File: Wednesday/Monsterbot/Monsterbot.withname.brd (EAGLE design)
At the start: 180 x 113 mm, 17 parts, among them U1_0_BRAIN ADAFRUIT-PRO-TRINKET-5V-BOB, U1_10_PENHOLDER_2 PENHOLDER, U1_11_PENHOLDER_3 PENHOLDER, U1_2_DISPLAY ADAFRUIT-1.2IN-8X8-LED-BACKPA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, U1_4_SERVO SERVOMICROSIDE, U1_5_CASTER CASTERADAFRUIT-3/4IN, U1_6_PENHOLDER PENHOLDER

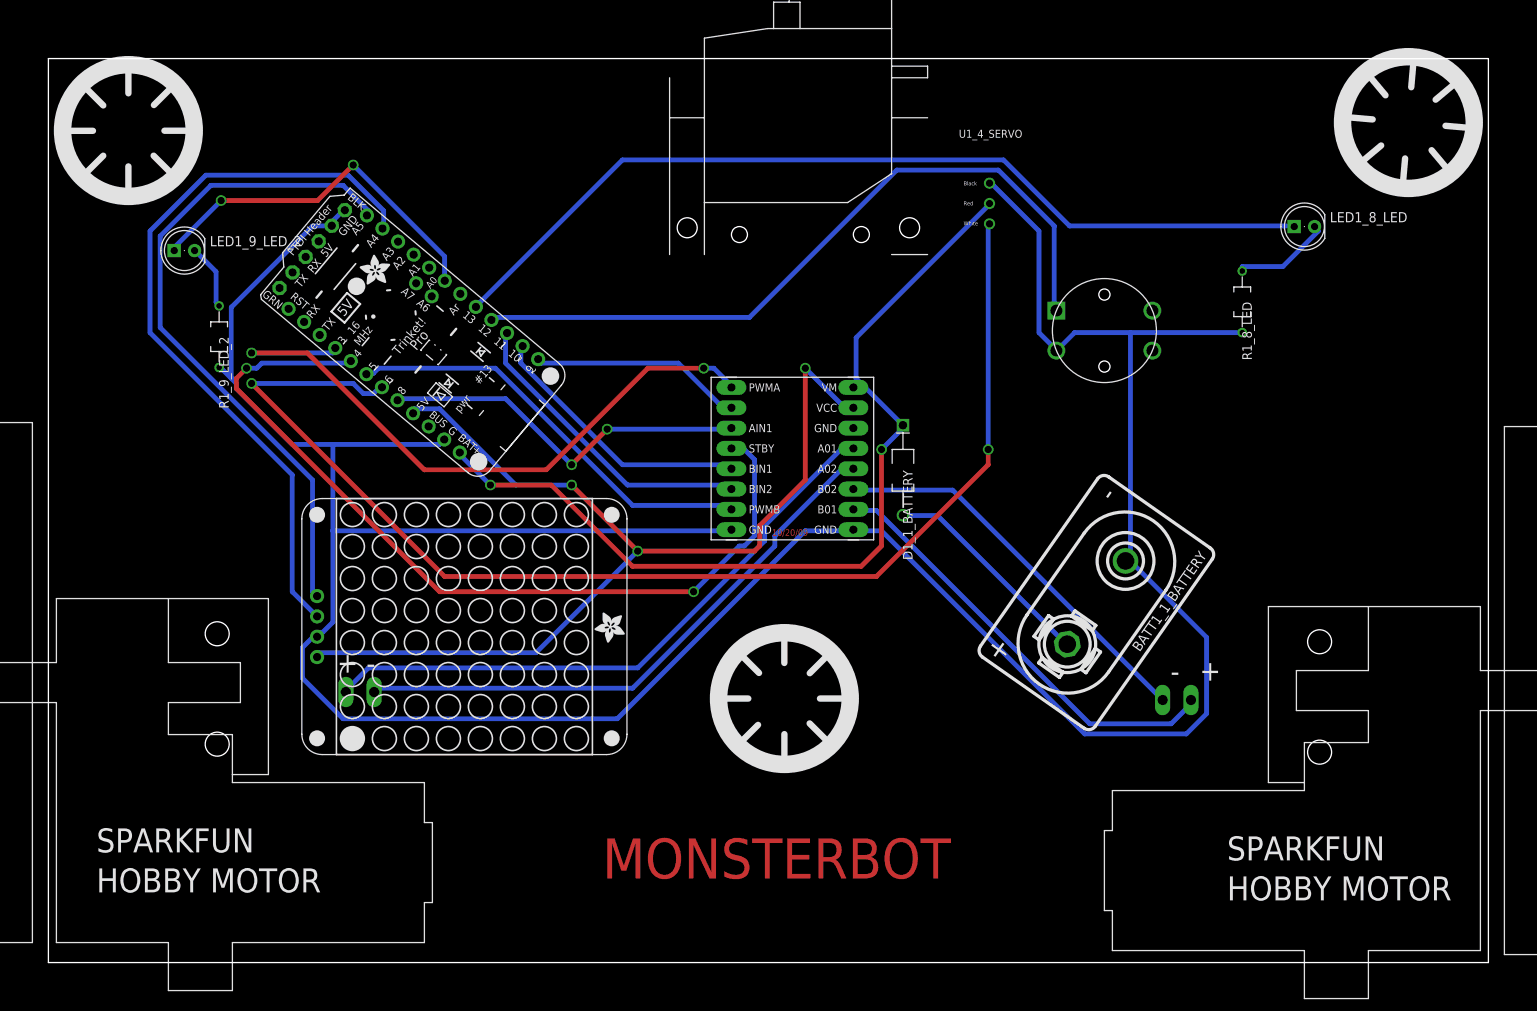
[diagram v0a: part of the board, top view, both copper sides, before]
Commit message: Readme
git-svn-id: svn+ssh://bbfs-01.calit2.net/grw/Gordon/svn/trunk/Gadgets/Designs/CSE91Robots@22925 2cf53259-273a-af40-bda6-69d31023b8ec
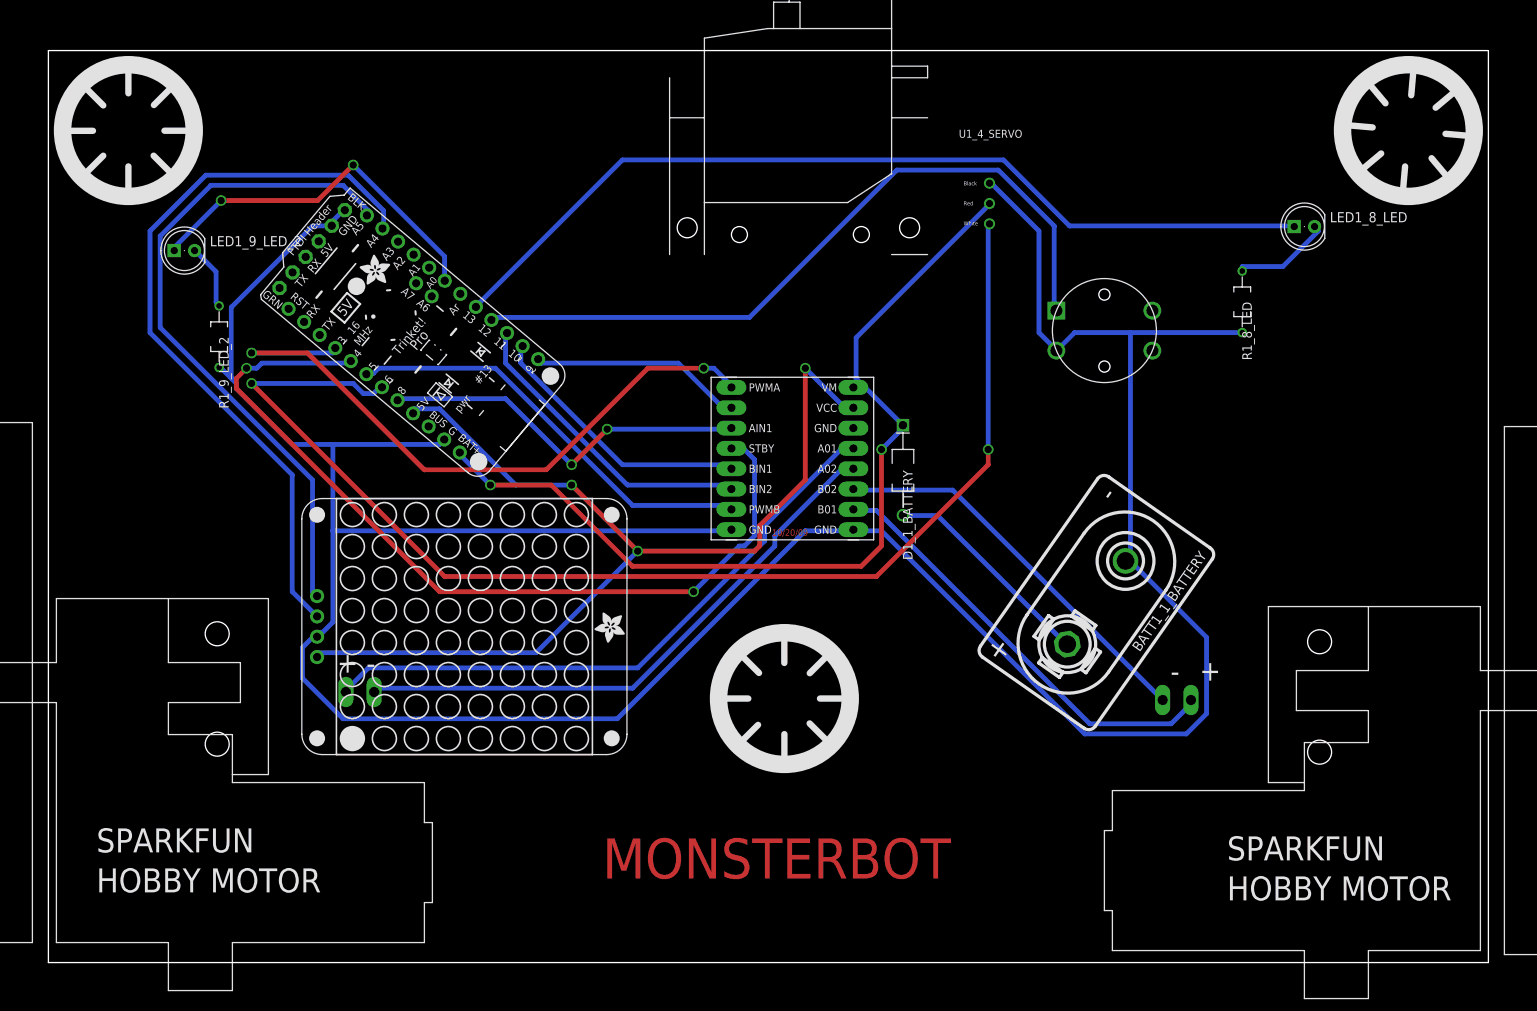
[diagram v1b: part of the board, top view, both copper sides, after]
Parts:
- moved U1_6_PENHOLDER 1.00 mm to (170.0, 104.0)
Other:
- board size 180 x 113 mm -> 180 x 114 mm
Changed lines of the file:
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@@
 <setting verticaltext="up"/>
 </settings>
-<grid distance="1" unitdist="mm" unit="mm" style="lines" multiple="1" display="no" altdistance="0.001" altunitdist="mm" altunit="mm"/>
+<grid distance="1" unitdist="mm" unit="mm" style="lines" multiple="1" display="yes" altdistance="0.001" altunitdist="mm" altunit="mm"/>
 <layers>
 <layer number="1" name="Top" color="4" fill="1" visible="yes" active="yes"/>
@@
 <plain>
 <rectangle x1="-30" y1="-5.005" x2="49.34" y2="69" layer="43"/>
-<wire x1="0" y1="0" x2="0" y2="113" width="0.1" layer="20"/>
-<wire x1="0" y1="113" x2="180" y2="113" width="0.1" layer="20"/>
+<wire x1="0" y1="0" x2="0" y2="114" width="0.1" layer="20"/>
+<wire x1="0" y1="114" x2="180" y2="114" width="0.1" layer="20"/>
 <rectangle x1="0.233121875" y1="94.233121875" x2="19.766878125" y2="113.766878125" layer="43"/>
 <circle x="100.62" y="54.11" radius="3.3796" width="0.001" layer="165"/>
@@
 <circle x="18.27" y="89" radius="2.3382" width="0.001" layer="164"/>
 <wire x1="180" y1="0" x2="0" y2="0" width="0.1" layer="20"/>
-<wire x1="180" y1="113" x2="180" y2="0" width="0.1" layer="20"/>
+<wire x1="180" y1="114" x2="180" y2="0" width="0.1" layer="20"/>
 <rectangle x1="19.89085625" y1="72.934075" x2="22.79085625" y2="75.834075" layer="41"/>
 <rectangle x1="19.89085625" y1="80.634075" x2="22.79085625" y2="83.534075" layer="41"/>
@@
 <element name="U1_4_SERVO" library="Components" package="SERVO_MICRO_SIDE" value="SERVOMICROSIDE" x="82" y="95" locked="yes"/>
 <element name="U1_5_CASTER" library="Components" package="ADAFRUIT-3/4IN-CASTER" value="CASTERADAFRUIT-3/4IN" x="94" y="91" locked="yes"/>
-<element name="U1_6_PENHOLDER" library="Components" package="PENHOLDER" value="PENHOLDER" x="170" y="105" locked="yes" rot="R310"/>
+<element name="U1_6_PENHOLDER" library="Components" package="PENHOLDER" value="PENHOLDER" x="170" y="104" rot="R310"/>
 </elements>
 <signals>
